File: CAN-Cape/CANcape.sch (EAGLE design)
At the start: 8 parts

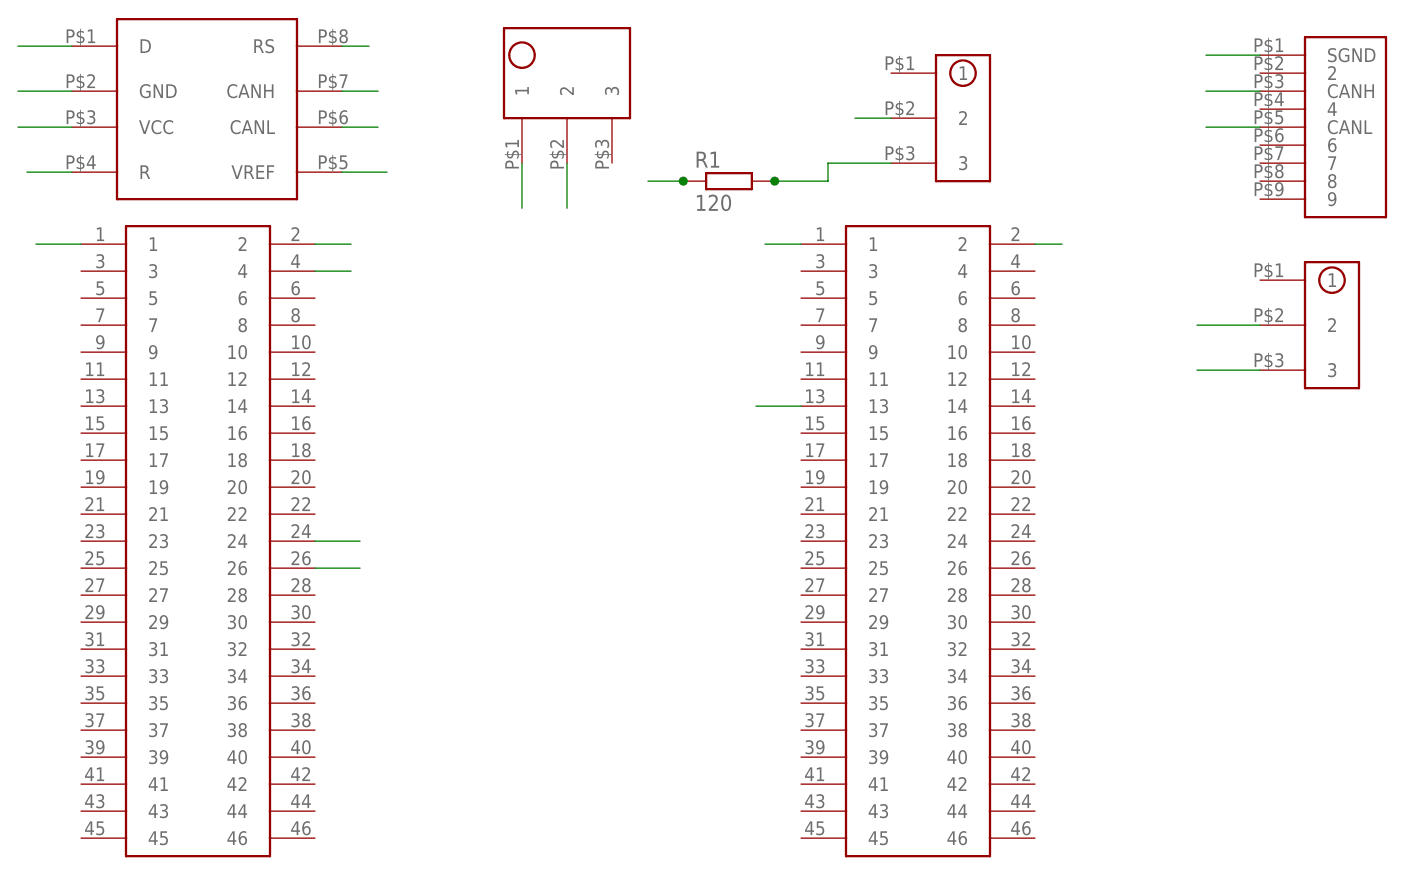
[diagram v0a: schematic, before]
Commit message: updated footprints and board design
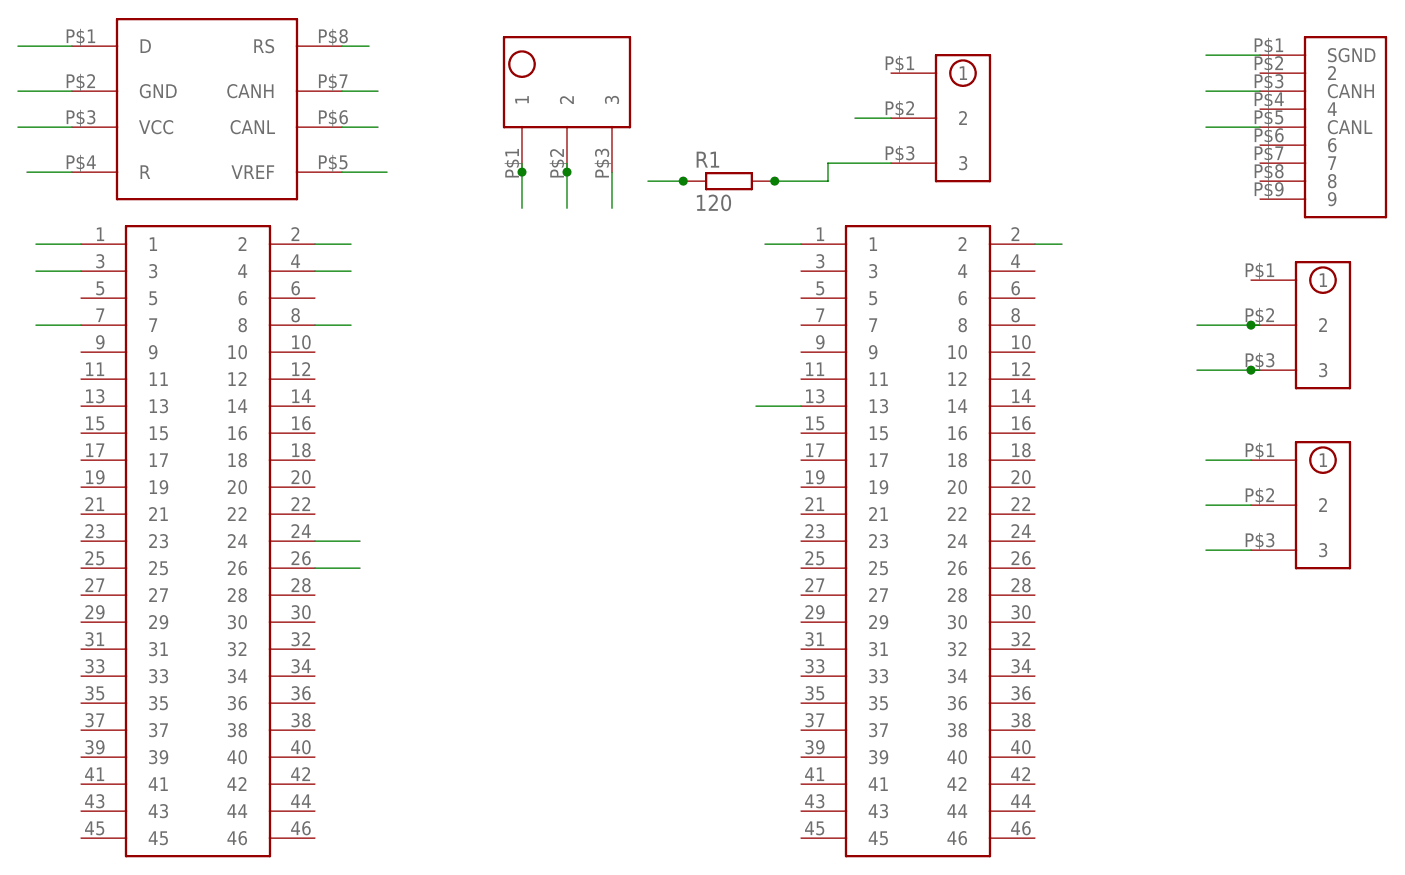
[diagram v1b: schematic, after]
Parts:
- added U$8: 1X3_HEADER, CANcape:1X3_HEADER
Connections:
- new net 5V: U$1.7, U$1.8, U$8.3
- new net TRAN_PWR: U$5.VCC, U$8.2
- net 3.3V: now also U$1.3, U$8.1; no longer U$5.VCC
- net SGND: now also U$3.3
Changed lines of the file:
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@@
 <part name="U$1" library="CANcape" deviceset="2X23_STACKABLE_HEADERS" device=""/>
 <part name="U$2" library="CANcape" deviceset="2X23_STACKABLE_HEADERS" device=""/>
-<part name="U$3" library="CANcape" deviceset="TB-5.0-PT-3P" device=""/>
-<part name="U$4" library="CANcape" deviceset="1X3_HEADER" device=""/>
-<part name="U$6" library="CANcape" deviceset="DB9_BREAKOUT" device=""/>
-<part name="U$7" library="CANcape" deviceset="1X3_HEADER" device=""/>
 <part name="U$5" library="SPST-switch" deviceset="SN65HVD320" device=""/>
 <part name="R1" library="resistor" deviceset="R-EU_" device="0207/15" value="120"/>
+<part name="U$3" library="CANcape" deviceset="TB-5.0-PT-3P" device=""/>
+<part name="U$6" library="CANcape" deviceset="DB9_BREAKOUT" device=""/>
+<part name="U$4" library="CANcape" deviceset="1X3_HEADER" device=""/>
+<part name="U$7" library="CANcape" deviceset="1X3_HEADER" device=""/>
+<part name="U$8" library="CANcape" deviceset="1X3_HEADER" device=""/>
 </parts>
 <sheets>
@@
 <instance part="U$1" gate="G$1" x="27" y="66"/>
 <instance part="U$2" gate="G$1" x="107" y="66"/>
-<instance part="U$3" gate="G$1" x="67" y="105" rot="R90"/>
-<instance part="U$4" gate="G$1" x="112" y="100"/>
-<instance part="U$6" gate="G$1" x="153" y="99"/>
-<instance part="U$7" gate="G$1" x="153" y="77"/>
 <instance part="U$5" gate="G$1" x="28" y="101"/>
 <instance part="R1" gate="G$1" x="86" y="93"/>
+<instance part="U$3" gate="G$1" x="67" y="104" rot="R90"/>
+<instance part="U$6" gate="G$1" x="153" y="99"/>
+<instance part="U$4" gate="G$1" x="112" y="100"/>
+<instance part="U$7" gate="G$1" x="152" y="77"/>
+<instance part="U$8" gate="G$1" x="152" y="57"/>
 </instances>
 <busses>
@@
 <net name="CANH" class="0">
 <segment>
+<wire x1="63" y1="95" x2="63" y2="94" width="0.1524" layer="91"/>
 <pinref part="U$3" gate="G$1" pin="1"/>
-<wire x1="63" y1="95" x2="63" y2="90" width="0.1524" layer="91"/>
+<wire x1="63" y1="94" x2="63" y2="90" width="0.1524" layer="91"/>
+<junction x="63" y="94"/>
 </segment>
 <segment>
+<wire x1="104" y1="100" x2="100" y2="100" width="0.1524" layer="91"/>
 <pinref part="U$4" gate="G$1" pin="2"/>
-<wire x1="104" y1="100" x2="100" y2="100" width="0.1524" layer="91"/>
 </segment>
 <segment>
@@
 </segment>
 <segment>
+<wire x1="145" y1="103" x2="139" y2="103" width="0.1524" layer="91"/>
 <pinref part="U$6" gate="G$1" pin="CANH"/>
-<wire x1="145" y1="103" x2="139" y2="103" width="0.1524" layer="91"/>
 </segment>
 </net>
 <net name="CANL" class="0">
 <segment>
+<wire x1="68" y1="95" x2="68" y2="94" width="0.1524" layer="91"/>
 <pinref part="U$3" gate="G$1" pin="2"/>
-<wire x1="68" y1="95" x2="68" y2="90" width="0.1524" layer="91"/>
+<wire x1="68" y1="94" x2="68" y2="90" width="0.1524" layer="91"/>
+<junction x="68" y="94"/>
 </segment>
 <segment>
@@
 </segment>
 <segment>
+<wire x1="145" y1="99" x2="139" y2="99" width="0.1524" layer="91"/>
 <pinref part="U$6" gate="G$1" pin="CANL"/>
-<wire x1="145" y1="99" x2="139" y2="99" width="0.1524" layer="91"/>
 </segment>
 <segment>
@@
 </segment>
 <segment>
+<wire x1="145" y1="72" x2="144" y2="72" width="0.1524" layer="91"/>
 <pinref part="U$7" gate="G$1" pin="3"/>
-<wire x1="145" y1="72" x2="138" y2="72" width="0.1524" layer="91"/>
+<wire x1="144" y1="72" x2="138" y2="72" width="0.1524" layer="91"/>
+<junction x="144" y="72"/>
 </segment>
 </net>
 <net name="3.3V" class="0">
-<segment>
-<wire x1="13" y1="99" x2="7" y2="99" width="0.1524" layer="91"/>
-<pinref part="U$5" gate="G$1" pin="VCC"/>
-</segment>
 <segment>
 <wire x1="43" y1="94" x2="48" y2="94" width="0.1524" layer="91"/>
@@
 <pinref part="U$1" gate="G$1" pin="4"/>
 <wire x1="40" y1="83" x2="44" y2="83" width="0.1524" layer="91"/>
+</segment>
+<segment>
+<pinref part="U$8" gate="G$1" pin="1"/>
+<wire x1="144" y1="62" x2="139" y2="62" width="0.1524" layer="91"/>
+</segment>
+<segment>
+<pinref part="U$1" gate="G$1" pin="3"/>
+<wire x1="14" y1="83" x2="9" y2="83" width="0.1524" layer="91"/>
 </segment>
 </net>
@@
 <wire x1="91.08" y1="93" x2="97" y2="93" width="0.1524" layer="91"/>
 <wire x1="97" y1="93" x2="97" y2="95" width="0.1524" layer="91"/>
-<pinref part="U$4" gate="G$1" pin="3"/>
 <wire x1="97" y1="95" x2="104" y2="95" width="0.1524" layer="91"/>
 <pinref part="R1" gate="G$1" pin="2"/>
 <junction x="91.08" y="93"/>
+<pinref part="U$4" gate="G$1" pin="3"/>
 </segment>
 </net>
 <net name="SGND" class="0">
 <segment>
+<wire x1="145" y1="77" x2="144" y2="77" width="0.1524" layer="91"/>
 <pinref part="U$7" gate="G$1" pin="2"/>
-<wire x1="145" y1="77" x2="138" y2="77" width="0.1524" layer="91"/>
+<wire x1="144" y1="77" x2="138" y2="77" width="0.1524" layer="91"/>
+<junction x="144" y="77"/>
 </segment>
 <segment>
+<wire x1="145" y1="107" x2="139" y2="107" width="0.1524" layer="91"/>
 <pinref part="U$6" gate="G$1" pin="SGND"/>
-<wire x1="145" y1="107" x2="139" y2="107" width="0.1524" layer="91"/>
+</segment>
+<segment>
+<pinref part="U$3" gate="G$1" pin="3"/>
+<wire x1="73" y1="94" x2="73" y2="90" width="0.1524" layer="91"/>
 </segment>
 </net>
+<net name="TRAN_PWR" class="0">
+<segment>
+<pinref part="U$5" gate="G$1" pin="VCC"/>
+<wire x1="13" y1="99" x2="7" y2="99" width="0.1524" layer="91"/>
+</segment>
+<segment>
+<pinref part="U$8" gate="G$1" pin="2"/>
+<wire x1="144" y1="57" x2="139" y2="57" width="0.1524" layer="91"/>
+</segment>
+</net>
+<net name="5V" class="0">
+<segment>
+<pinref part="U$8" gate="G$1" pin="3"/>
+<wire x1="144" y1="52" x2="139" y2="52" width="0.1524" layer="91"/>
+</segment>
+<segment>
+<pinref part="U$1" gate="G$1" pin="7"/>
+<wire x1="14" y1="77" x2="9" y2="77" width="0.1524" layer="91"/>
+</segment>
+<segment>
+<pinref part="U$1" gate="G$1" pin="8"/>
+<wire x1="40" y1="77" x2="44" y2="77" width="0.1524" layer="91"/>
+</segment>
+</net>

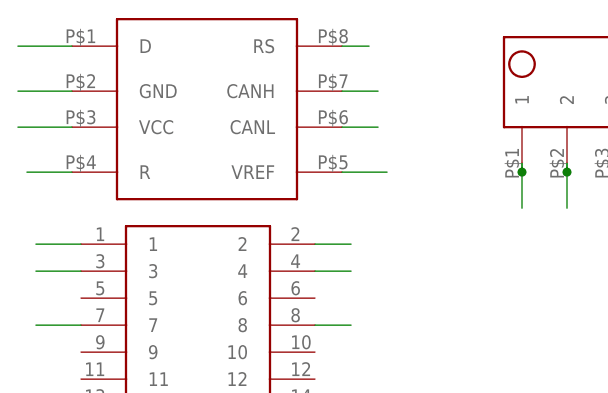
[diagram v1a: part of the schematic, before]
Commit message: more board work
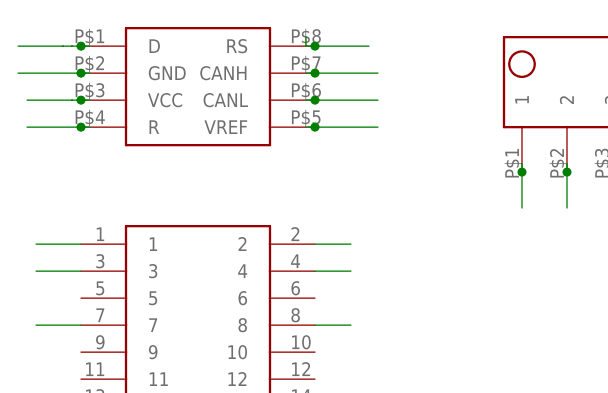
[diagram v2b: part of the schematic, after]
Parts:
- U$5: value SN65HVD320 -> SOIC_BREAKOUT; device SPST-switch:SN65HVD320 -> CANcape:SOIC_BREAKOUT
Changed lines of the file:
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@@
 <part name="U$1" library="CANcape" deviceset="2X23_STACKABLE_HEADERS" device=""/>
 <part name="U$2" library="CANcape" deviceset="2X23_STACKABLE_HEADERS" device=""/>
-<part name="U$5" library="SPST-switch" deviceset="SN65HVD320" device=""/>
 <part name="R1" library="resistor" deviceset="R-EU_" device="0207/15" value="120"/>
 <part name="U$3" library="CANcape" deviceset="TB-5.0-PT-3P" device=""/>
@@
 <part name="U$7" library="CANcape" deviceset="1X3_HEADER" device=""/>
 <part name="U$8" library="CANcape" deviceset="1X3_HEADER" device=""/>
+<part name="U$5" library="CANcape" deviceset="SOIC_BREAKOUT" device=""/>
 </parts>
 <sheets>
@@
 <instance part="U$1" gate="G$1" x="27" y="66"/>
 <instance part="U$2" gate="G$1" x="107" y="66"/>
-<instance part="U$5" gate="G$1" x="28" y="101"/>
 <instance part="R1" gate="G$1" x="86" y="93"/>
 <instance part="U$3" gate="G$1" x="67" y="104" rot="R90"/>
@@
 <instance part="U$7" gate="G$1" x="152" y="77"/>
 <instance part="U$8" gate="G$1" x="152" y="57"/>
+<instance part="U$5" gate="G$1" x="27" y="103"/>
 </instances>
 <busses>
@@
 </segment>
 <segment>
-<wire x1="13" y1="94" x2="8" y2="94" width="0.1524" layer="91"/>
+<wire x1="15" y1="99" x2="14" y2="99" width="0.1524" layer="91"/>
 <pinref part="U$5" gate="G$1" pin="R"/>
+<wire x1="14" y1="99" x2="8" y2="99" width="0.1524" layer="91"/>
+<junction x="14" y="99"/>
 </segment>
 </net>
@@
 </segment>
 <segment>
-<wire x1="13" y1="108" x2="7" y2="108" width="0.1524" layer="91"/>
+<wire x1="13" y1="108" x2="12" y2="108" width="0.1524" layer="91"/>
+<wire x1="12" y1="108" x2="7" y2="108" width="0.1524" layer="91"/>
+<wire x1="15" y1="108" x2="14" y2="108" width="0.1524" layer="91"/>
 <pinref part="U$5" gate="G$1" pin="D"/>
+<wire x1="14" y1="108" x2="13" y2="108" width="0.1524" layer="91"/>
+<junction x="14" y="108"/>
 </segment>
 </net>
@@
 </segment>
 <segment>
-<wire x1="43" y1="103" x2="47" y2="103" width="0.1524" layer="91"/>
+<wire x1="47" y1="105" x2="40" y2="105" width="0.1524" layer="91"/>
 <pinref part="U$5" gate="G$1" pin="CANH"/>
+<wire x1="40" y1="105" x2="39" y2="105" width="0.1524" layer="91"/>
+<junction x="40" y="105"/>
 </segment>
 <segment>
@@
 </segment>
 <segment>
-<wire x1="43" y1="99" x2="47" y2="99" width="0.1524" layer="91"/>
+<wire x1="47" y1="102" x2="40" y2="102" width="0.1524" layer="91"/>
 <pinref part="U$5" gate="G$1" pin="CANL"/>
+<wire x1="40" y1="102" x2="39" y2="102" width="0.1524" layer="91"/>
+<junction x="40" y="102"/>
 </segment>
 <segment>
@@
 </segment>
 <segment>
-<wire x1="13" y1="103" x2="7" y2="103" width="0.1524" layer="91"/>
+<wire x1="15" y1="105" x2="14" y2="105" width="0.1524" layer="91"/>
 <pinref part="U$5" gate="G$1" pin="GND"/>
+<wire x1="14" y1="105" x2="7" y2="105" width="0.1524" layer="91"/>
+<junction x="14" y="105"/>
 </segment>
 <segment>
@@
 <net name="3.3V" class="0">
 <segment>
-<wire x1="43" y1="94" x2="48" y2="94" width="0.1524" layer="91"/>
+<wire x1="39" y1="99" x2="40" y2="99" width="0.1524" layer="91"/>
 <pinref part="U$5" gate="G$1" pin="VREF"/>
+<wire x1="40" y1="99" x2="47" y2="99" width="0.1524" layer="91"/>
+<junction x="40" y="99"/>
 </segment>
 <segment>
@@
 <net name="STANDBY" class="0">
 <segment>
-<wire x1="43" y1="108" x2="46" y2="108" width="0.1524" layer="91"/>
+<wire x1="46" y1="108" x2="40" y2="108" width="0.1524" layer="91"/>
+<wire x1="40" y1="108" x2="39" y2="108" width="0.1524" layer="91"/>
+<wire x1="39" y1="108" x2="39" y2="109" width="0.1524" layer="91"/>
 <pinref part="U$5" gate="G$1" pin="RS"/>
+<junction x="40" y="108"/>
 </segment>
 <segment>
@@
 <net name="TRAN_PWR" class="0">
 <segment>
+<wire x1="14" y1="102" x2="13" y2="102" width="0.1524" layer="91"/>
+<wire x1="13" y1="102" x2="8" y2="102" width="0.1524" layer="91"/>
+<wire x1="15" y1="102" x2="14" y2="102" width="0.1524" layer="91"/>
 <pinref part="U$5" gate="G$1" pin="VCC"/>
-<wire x1="13" y1="99" x2="7" y2="99" width="0.1524" layer="91"/>
+<junction x="14" y="102"/>
 </segment>
 <segment>
